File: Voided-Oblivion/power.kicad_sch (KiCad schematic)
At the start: 133 parts, among them Q1 AO3401, Q10 BC847B, Q11 BC847B, Q13 NCE4009S, Q14 NCE4009S, Q2 AO4407A, Q3 BC857, Q4 AO4407A, Q5 AO4407A, Q6 AO4407A, Q7 AO4407A, Q8 BC847B, Q9 BC847B, U10 TLV431BQDBZR, U11 LM2903, U12 AP2171WG-7, U13 TPD2E2U06DRL, U14 TPD2E2U06DRL, U15 LM66100DCKT, U16 AP2171WG-7, U17 LM74700QDDF, U18 LM74700QDDF, U2 TS3USB30ERSWR, U5 TPS54302, U6 TPS54302, U7 TLV76733DRVR, U9 LM66100DCKT

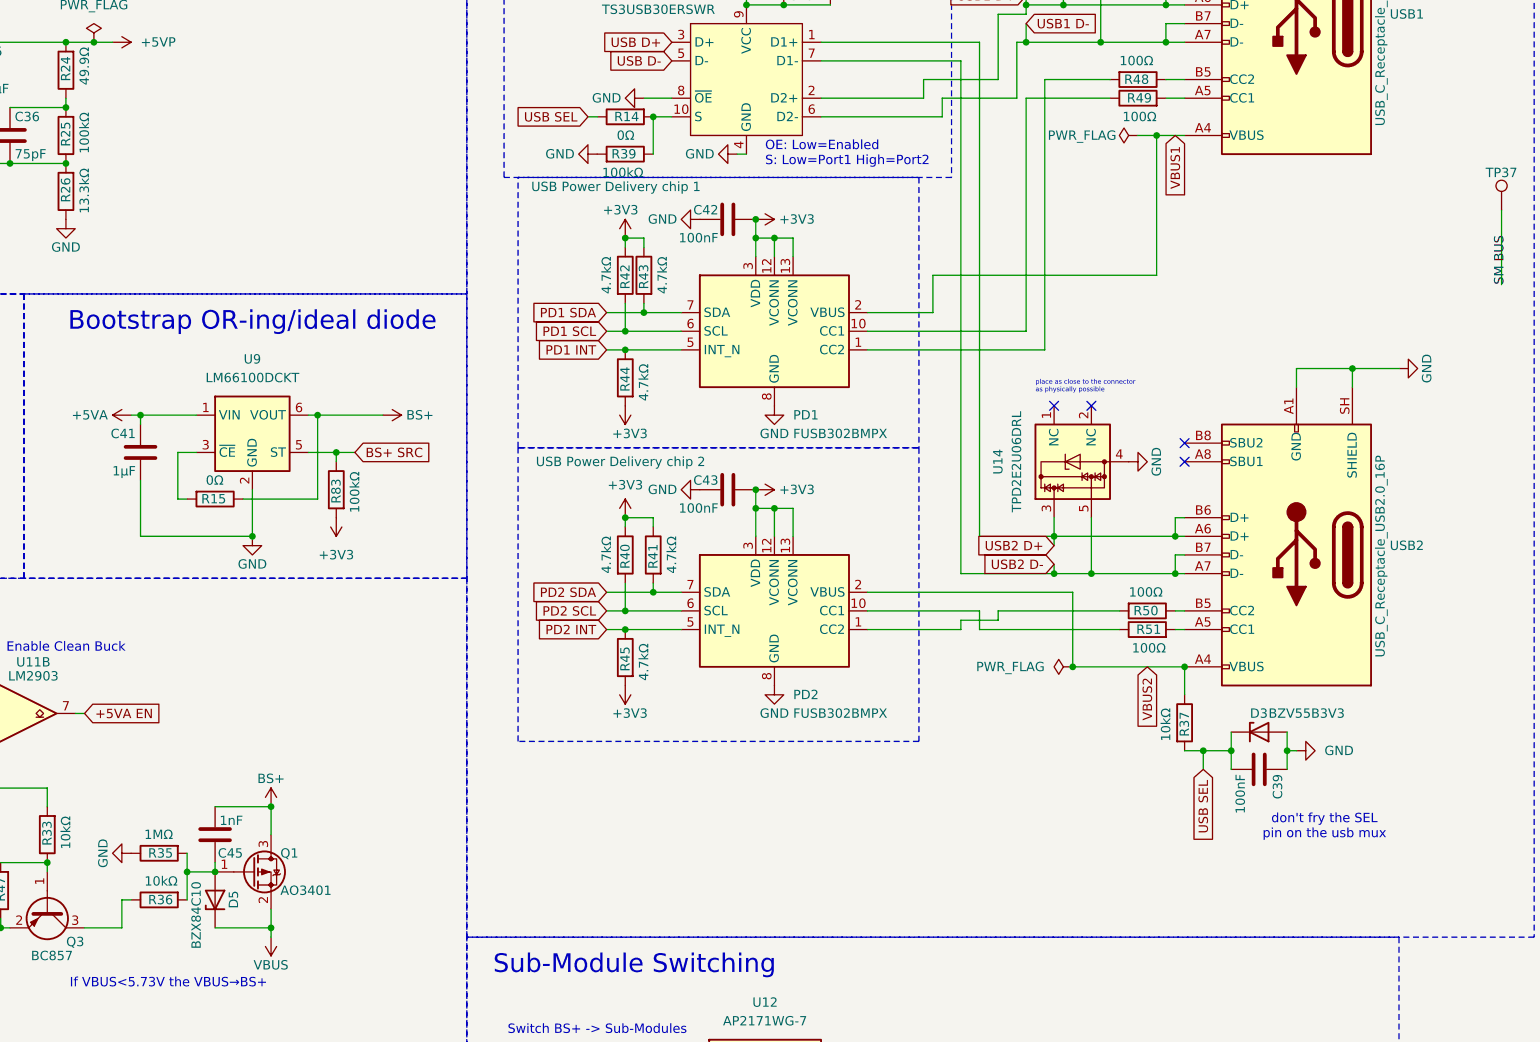
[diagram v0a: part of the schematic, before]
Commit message: small changes
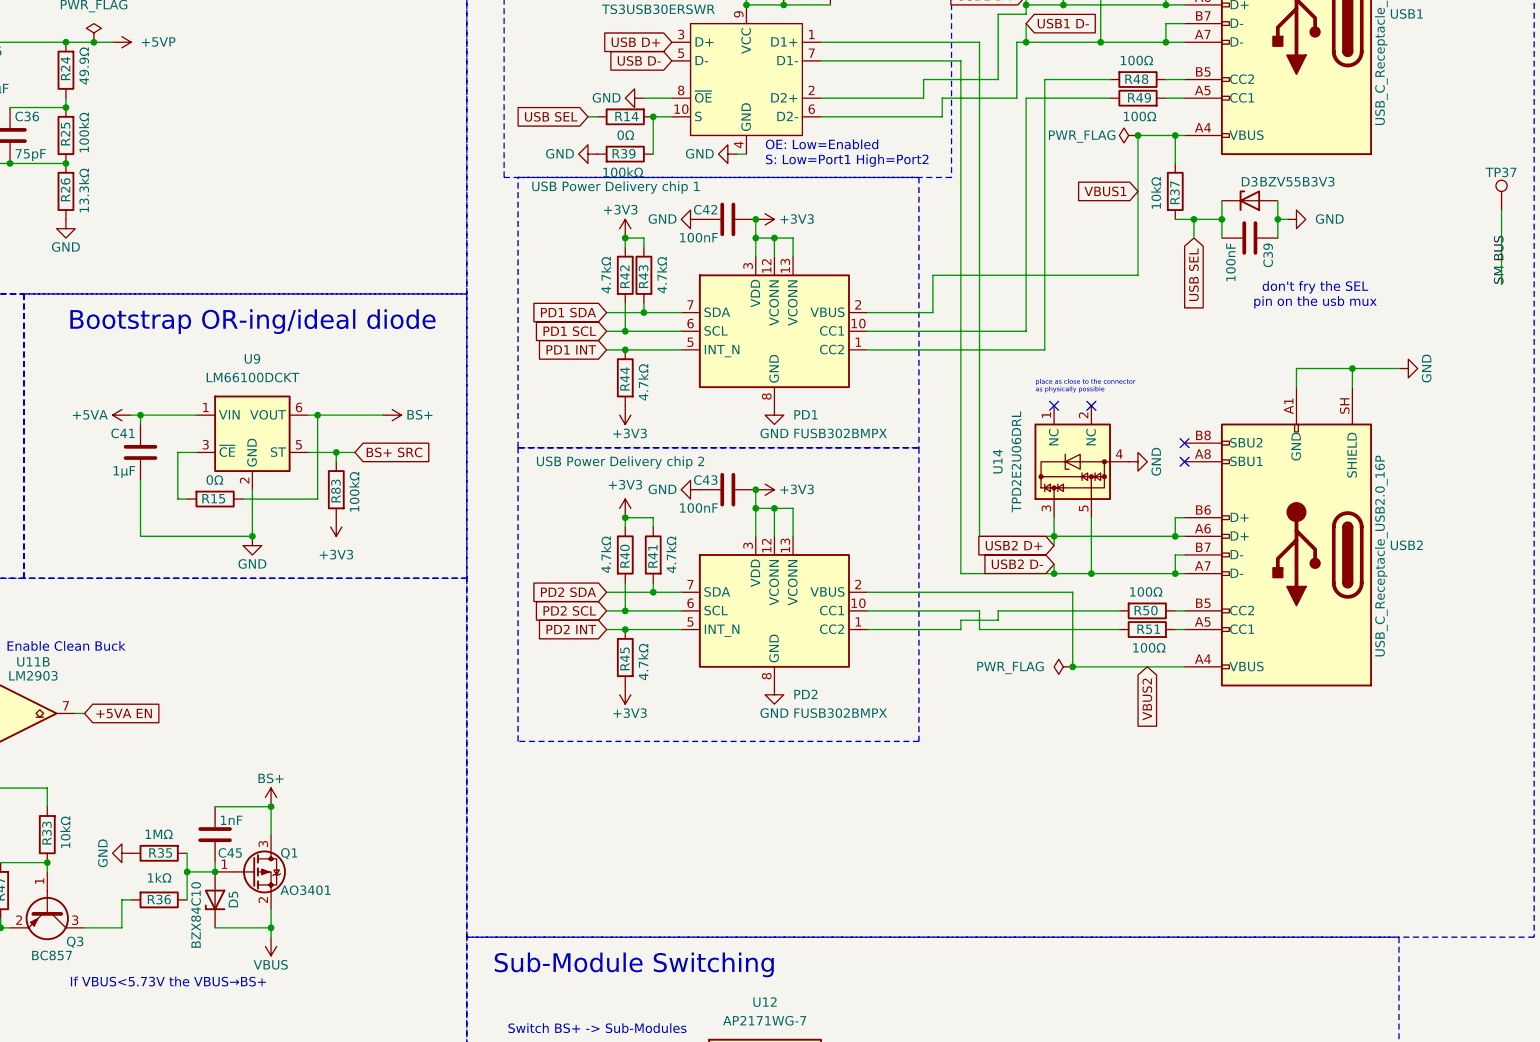
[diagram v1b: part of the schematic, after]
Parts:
- C114, C115, C116, C117, C118, C119, C120, C127, C128, C129, C130, C23, C24, C25, C27, C30, C32, C33, C36, C37, C38, C39, C41, C42, C43, C44, C45, C76: footprint Capacitor_SMD:C_0402_1005Metric -> Voided-Oblivion-misc:C_0402_1005Metric-no-silkscreen-text
- R102, R103, R12, R14, R15, R16, R18, R19, R20, R21, R22, R24, R25, R26, R27, R28, R29, R32, R33, R34, R35, R37, R38, R39, R40, R41, R42, R43, R44, R45, R46, R47, R48, R49, R50, R51, R67, R68, R69, R70, R71, R72, R73, R74, R75, R76, R77, R78, R79, R80, R81, R82, R83, R92, R95, R96: footprint Resistor_SMD:R_0402_1005Metric -> Voided-Oblivion-misc:R_0402_1005Metric-no-silkscreen-text
- R30: footprint Resistor_SMD:R_0402_1005Metric -> Voided-Oblivion-misc:R_0402_1005Metric-no-silkscreen-text; MPN ARG02BTC4422 -> ARG02BTC3572
- R31: footprint Resistor_SMD:R_0402_1005Metric -> Voided-Oblivion-misc:R_0402_1005Metric-no-silkscreen-text; MPN (none) -> ARG02BTC1002
- R36: value 10kΩ -> 1kΩ; footprint Resistor_SMD:R_0402_1005Metric -> Voided-Oblivion-misc:R_0402_1005Metric-no-silkscreen-text; LCSC C25744 -> C11702; MPN 0402WGF1002TCE -> 0402WGF1001TCE
- U10: symbol Reference_Voltage:TL431DBZ -> Voided-Oblivion-misc:TL431BQDBZ
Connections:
- net +1V24ref: now also U10.2 (K); no longer U10.1 (K)
- net VBUS1: now also R37.1
- net VBUS2: no longer R37.1
- net at R27.1, R28.2: now also U10.1 (REF); no longer U10.2 (REF)
- net at Q3.3 (C): now also R36.2; no longer R36.1
- net at C45.1, D5.1 (A), Q1.1 (G)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: now also R36.1; no longer R36.2
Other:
- moved on the sheet: C39, D3, R37
